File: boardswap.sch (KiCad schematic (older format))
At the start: 154 parts, among them J1 USB_C_Receptacle_USB2.0, SW1 SW_Push, U1 ATmega32U4-AU, Y1 16MHz

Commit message: did most placement
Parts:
- C7: footprint Diode_SMD:D_SOD-123 -> Capacitor_SMD:C_0805_2012Metric
- J1: footprint keyswitches:Kailh_socket_MX -> Connector_USB:USB_C_Receptacle_HRO_TYPE-C-31-M-12
- U1: footprint Package_QFP:TQFP-44_10x10mm_P0.8mm -> Package_DFN_QFN:QFN-44-1EP_7x7mm_P0.5mm_EP5.2x5.2mm
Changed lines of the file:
@@
 F 0 "J1" H 1307 7367 50  0000 C CNN
 F 1 "USB_C_Receptacle_USB2.0" H 1307 7276 50  0000 C CNN
-F 2 "keyswitches:Kailh_socket_MX" H 1350 6500 50  0001 C CNN
+F 2 "Connector_USB:USB_C_Receptacle_HRO_TYPE-C-31-M-12" H 1350 6500 50  0001 C CNN
 F 3 "https://www.usb.org/sites/default/files/documents/usb_type-c.zip" H 1350 6500 50  0001 C CNN
 	1    1200 6500
@@
 F 0 "C7" H 2042 3746 50  0000 L CNN
 F 1 "10uF" H 2042 3655 50  0000 L CNN
-F 2 "Diode_SMD:D_SOD-123" H 1950 3700 50  0001 C CNN
+F 2 "Capacitor_SMD:C_0805_2012Metric" H 1950 3700 50  0001 C CNN
 F 3 "~" H 1950 3700 50  0001 C CNN
 	1    1950 3700
@@
 F 0 "U1" H 3400 1111 50  0000 C CNN
 F 1 "ATmega32U4-AU" H 3400 1020 50  0000 C CNN
-F 2 "Package_QFP:TQFP-44_10x10mm_P0.8mm" H 3400 3000 50  0001 C CIN
+F 2 "Package_DFN_QFN:QFN-44-1EP_7x7mm_P0.5mm_EP5.2x5.2mm" H 3400 3000 50  0001 C CIN
 F 3 "http://ww1.microchip.com/downloads/en/DeviceDoc/Atmel-7766-8-bit-AVR-ATmega16U4-32U4_Datasheet.pdf" H 3400 3000 50  0001 C CNN
 	1    3400 3000

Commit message: hewwo backups owo
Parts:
- U1: footprint Package_DFN_QFN:QFN-44-1EP_7x7mm_P0.5mm_EP5.2x5.2mm -> Package_QFP:TQFP-44_10x10mm_P0.8mm
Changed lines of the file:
@@
 F 0 "U1" H 3400 1111 50  0000 C CNN
 F 1 "ATmega32U4-AU" H 3400 1020 50  0000 C CNN
-F 2 "Package_DFN_QFN:QFN-44-1EP_7x7mm_P0.5mm_EP5.2x5.2mm" H 3400 3000 50  0001 C CIN
+F 2 "Package_QFP:TQFP-44_10x10mm_P0.8mm" H 3400 3000 50  0001 C CIN
 F 3 "http://ww1.microchip.com/downloads/en/DeviceDoc/Atmel-7766-8-bit-AVR-ATmega16U4-32U4_Datasheet.pdf" H 3400 3000 50  0001 C CNN
 	1    3400 3000

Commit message: placed components
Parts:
- C4, C5, C6, C7: footprint Capacitor_SMD:C_0805_2012Metric -> Capacitor_SMD:C_0603_1608Metric
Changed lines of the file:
@@
 	1    0    0    -1
 $EndComp
-Connection ~ 2800 1500
 Wire Wire Line
 	2300 1500 2300 1200
@@
 	1    0    0    -1
 $EndComp
-Wire Wire Line
-	2800 1500 2800 1250
 $Comp
 L Device:R_Small R1
@@
 F 0 "C7" H 2042 3746 50  0000 L CNN
 F 1 "10uF" H 2042 3655 50  0000 L CNN
-F 2 "Capacitor_SMD:C_0805_2012Metric" H 1950 3700 50  0001 C CNN
+F 2 "Capacitor_SMD:C_0603_1608Metric" H 1950 3700 50  0001 C CNN
 F 3 "~" H 1950 3700 50  0001 C CNN
 	1    1950 3700
@@
 F 0 "C6" H 1642 3746 50  0000 L CNN
 F 1 "0.1uF" H 1642 3655 50  0000 L CNN
-F 2 "Capacitor_SMD:C_0805_2012Metric" H 1550 3700 50  0001 C CNN
+F 2 "Capacitor_SMD:C_0603_1608Metric" H 1550 3700 50  0001 C CNN
 F 3 "~" H 1550 3700 50  0001 C CNN
 	1    1550 3700
@@
 F 0 "C5" H 1242 3746 50  0000 L CNN
 F 1 "0.1uF" H 1242 3655 50  0000 L CNN
-F 2 "Capacitor_SMD:C_0805_2012Metric" H 1150 3700 50  0001 C CNN
+F 2 "Capacitor_SMD:C_0603_1608Metric" H 1150 3700 50  0001 C CNN
 F 3 "~" H 1150 3700 50  0001 C CNN
 	1    1150 3700
@@
 F 0 "C4" H 842 3746 50  0000 L CNN
 F 1 "0.1uF" H 842 3655 50  0000 L CNN
-F 2 "Capacitor_SMD:C_0805_2012Metric" H 750 3700 50  0001 C CNN
+F 2 "Capacitor_SMD:C_0603_1608Metric" H 750 3700 50  0001 C CNN
 F 3 "~" H 750 3700 50  0001 C CNN
 	1    750  3700
@@
 $EndComp
 Wire Wire Line
-	3300 4800 2950 4800
-Connection ~ 3300 4800
-Wire Wire Line
-	2950 4800 2950 4900
-Wire Wire Line
-	3400 4800 3300 4800
-$Comp
-L power:GND #PWR0109
-U 1 1 5F31D09C
-P 2950 4900
-F 0 "#PWR0109" H 2950 4650 50  0001 C CNN
-F 1 "GND" H 2955 4727 50  0000 C CNN
-F 2 "" H 2950 4900 50  0001 C CNN
-F 3 "" H 2950 4900 50  0001 C CNN
-	1    2950 4900
-	1    0    0    -1
-$EndComp
-Wire Wire Line
-	3400 1200 3400 1050
-Wire Wire Line
 	3400 1200 3500 1200
 Connection ~ 3400 1200
@@
 F 3 "" H 3400 1050 50  0001 C CNN
 	1    3400 1050
-	1    0    0    -1
-$EndComp
-$Comp
-L MCU_Microchip_ATmega:ATmega32U4-AU U1
-U 1 1 5F319131
-P 3400 3000
-F 0 "U1" H 3400 1111 50  0000 C CNN
-F 1 "ATmega32U4-AU" H 3400 1020 50  0000 C CNN
-F 2 "Package_QFP:TQFP-44_10x10mm_P0.8mm" H 3400 3000 50  0001 C CIN
-F 3 "http://ww1.microchip.com/downloads/en/DeviceDoc/Atmel-7766-8-bit-AVR-ATmega16U4-32U4_Datasheet.pdf" H 3400 3000 50  0001 C CNN
-	1    3400 3000
 	1    0    0    -1
 $EndComp
@@
 Text GLabel 10500 1200 1    50   Input ~ 0
 COL13
+Wire Wire Line
+	3400 1200 3400 1050
+Wire Wire Line
+	2800 1500 2800 1250
+$Comp
+L power:GND #PWR0109
+U 1 1 5F31D09C
+P 2950 4900
+F 0 "#PWR0109" H 2950 4650 50  0001 C CNN
+F 1 "GND" H 2955 4727 50  0000 C CNN
+F 2 "" H 2950 4900 50  0001 C CNN
+F 3 "" H 2950 4900 50  0001 C CNN
+	1    2950 4900
+	1    0    0    -1
+$EndComp
+Connection ~ 2800 1500
+Wire Wire Line
+	2950 4800 2950 4900
+$Comp
+L MCU_Microchip_ATmega:ATmega32U4-AU U1
+U 1 1 5F319131
+P 3400 3000
+F 0 "U1" H 3400 1111 50  0000 C CNN
+F 1 "ATmega32U4-AU" H 3400 1020 50  0000 C CNN
+F 2 "Package_QFP:TQFP-44_10x10mm_P0.8mm" H 3400 3000 50  0001 C CIN
+F 3 "http://ww1.microchip.com/downloads/en/DeviceDoc/Atmel-7766-8-bit-AVR-ATmega16U4-32U4_Datasheet.pdf" H 3400 3000 50  0001 C CNN
+	1    3400 3000
+	1    0    0    -1
+$EndComp
+Wire Wire Line
+	3400 4800 3300 4800
+Connection ~ 3300 4800
+Wire Wire Line
+	2950 4800 3300 4800
 $EndSCHEMATC

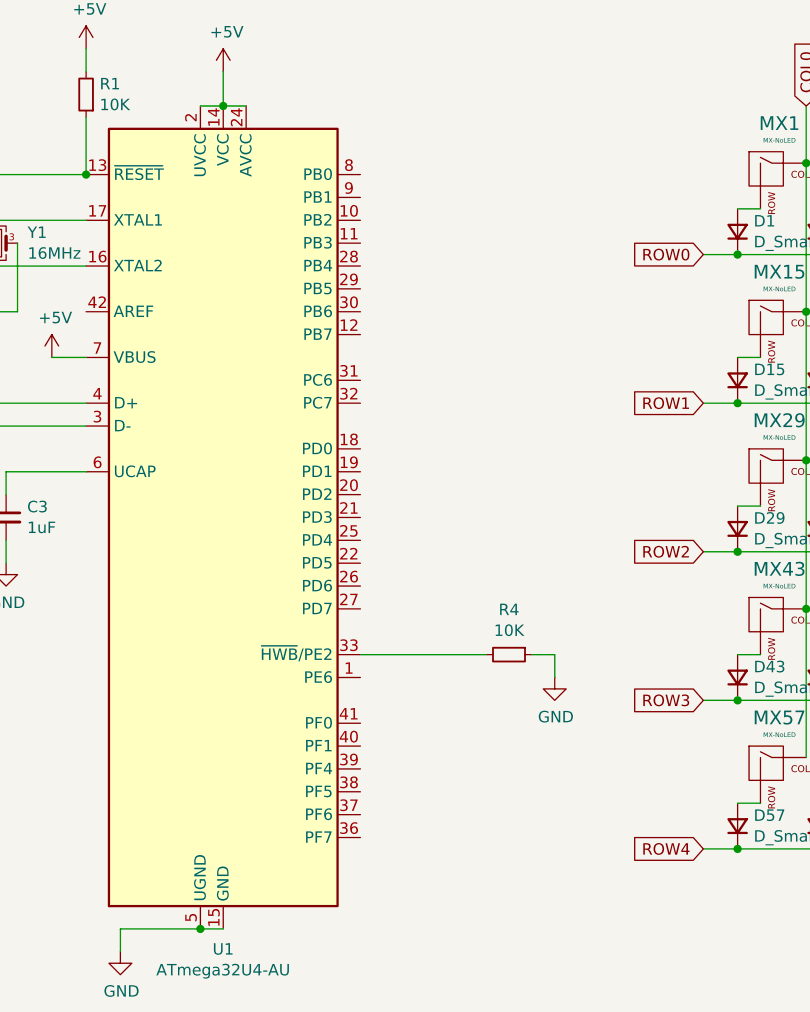
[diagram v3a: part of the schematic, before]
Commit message: done routing probably
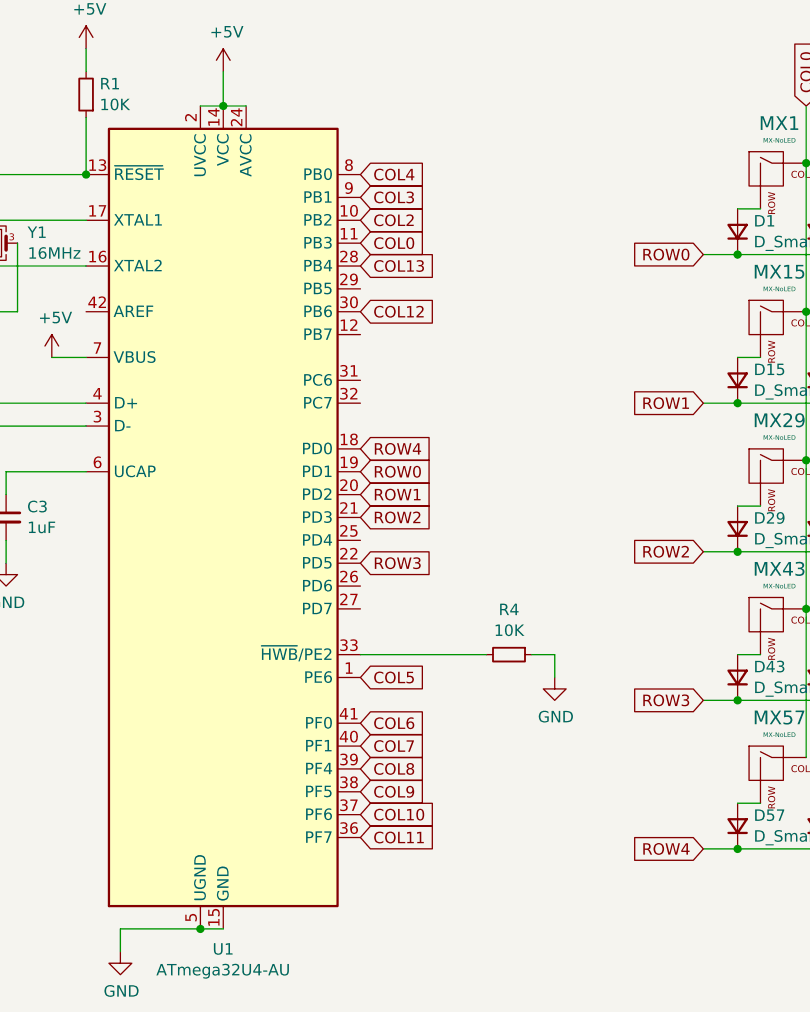
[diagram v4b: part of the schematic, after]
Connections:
- net COL0: now also U1.11 (PB3)
- net COL10: now also U1.37 (PF6)
- net COL11: now also U1.36 (PF7)
- net COL12: now also U1.30 (PB6)
- net COL13: now also U1.28 (PB4)
- net COL2: now also U1.10 (PB2)
- net COL3: now also U1.9 (PB1)
- net COL4: now also U1.8 (PB0)
- net COL5: now also U1.1 (PE6)
- net COL6: now also U1.41 (PF0)
- net COL7: now also U1.40 (PF1)
- net COL8: now also U1.39 (PF4)
- net COL9: now also U1.38 (PF5)
- net ROW0: now also U1.19 (PD1)
- net ROW1: now also U1.20 (PD2)
- net ROW2: now also U1.21 (PD3)
- net ROW3: now also U1.22 (PD5)
- net ROW4: now also U1.18 (PD0)
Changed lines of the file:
@@
 Wire Wire Line
 	2950 4800 3300 4800
+Text GLabel 4000 3200 2    50   Input ~ 0
+ROW3
+Text GLabel 4000 3000 2    50   Input ~ 0
+ROW2
+Text GLabel 4000 2900 2    50   Input ~ 0
+ROW1
+Text GLabel 4000 2800 2    50   Input ~ 0
+ROW0
+Text GLabel 4000 2700 2    50   Input ~ 0
+ROW4
+Text GLabel 4000 1800 2    50   Input ~ 0
+COL0
+Text GLabel 4000 1700 2    50   Input ~ 0
+COL2
+Text GLabel 4000 1600 2    50   Input ~ 0
+COL3
+Text GLabel 4000 1500 2    50   Input ~ 0
+COL4
+Text GLabel 4000 3700 2    50   Input ~ 0
+COL5
+Text GLabel 4000 3900 2    50   Input ~ 0
+COL6
+Text GLabel 4000 4000 2    50   Input ~ 0
+COL7
+Text GLabel 4000 4100 2    50   Input ~ 0
+COL8
+Text GLabel 4000 4200 2    50   Input ~ 0
+COL9
+Text GLabel 4000 4300 2    50   Input ~ 0
+COL10
+Text GLabel 4000 4400 2    50   Input ~ 0
+COL11
+Text GLabel 4000 2100 2    50   Input ~ 0
+COL12
+Text GLabel 4000 1900 2    50   Input ~ 0
+COL13
 $EndSCHEMATC

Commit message: rotated mcu, begrudgingly
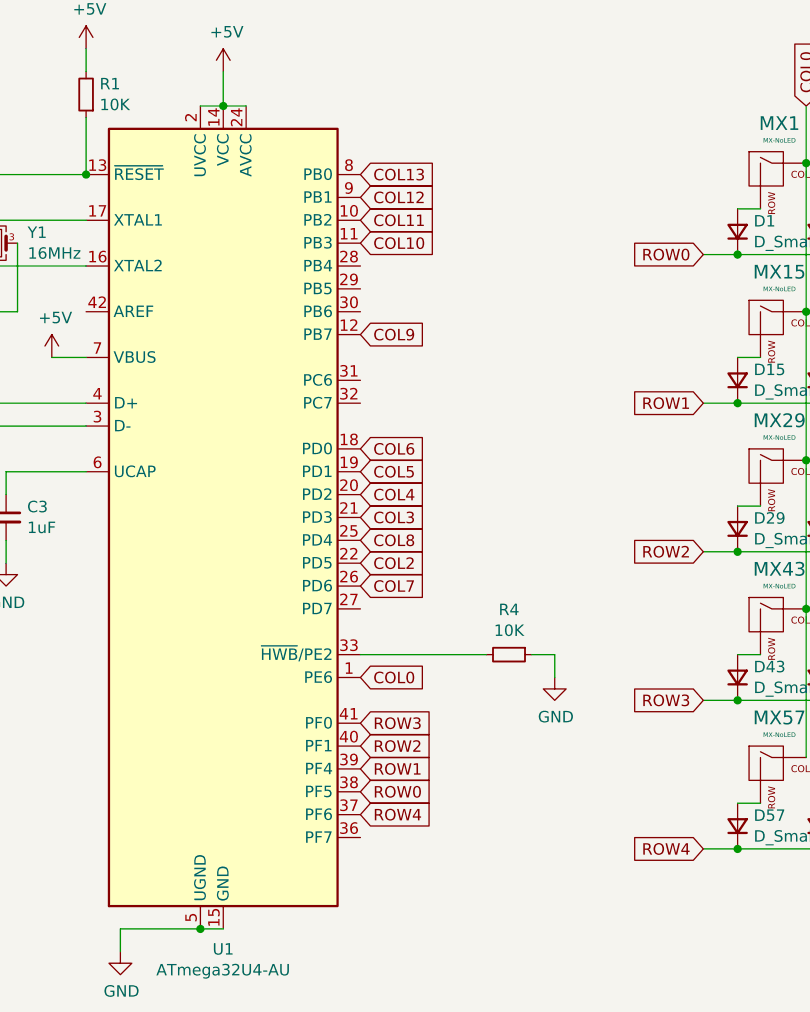
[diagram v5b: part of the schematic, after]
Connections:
- net COL0: now also U1.1 (PE6); no longer U1.11 (PB3)
- net COL10: now also U1.11 (PB3); no longer U1.37 (PF6)
- net COL11: now also U1.10 (PB2); no longer U1.36 (PF7)
- net COL12: now also U1.9 (PB1); no longer U1.30 (PB6)
- net COL13: now also U1.8 (PB0); no longer U1.28 (PB4)
- net COL2: now also U1.22 (PD5); no longer U1.10 (PB2)
- net COL3: now also U1.21 (PD3); no longer U1.9 (PB1)
- net COL4: now also U1.20 (PD2); no longer U1.8 (PB0)
- net COL5: now also U1.19 (PD1); no longer U1.1 (PE6)
- net COL6: now also U1.18 (PD0); no longer U1.41 (PF0)
- net COL7: now also U1.26 (PD6); no longer U1.40 (PF1)
- net COL8: now also U1.25 (PD4); no longer U1.39 (PF4)
- net COL9: now also U1.12 (PB7); no longer U1.38 (PF5)
- net ROW0: now also U1.38 (PF5); no longer U1.19 (PD1)
- net ROW1: now also U1.39 (PF4); no longer U1.20 (PD2)
- net ROW2: now also U1.40 (PF1); no longer U1.21 (PD3)
- net ROW3: now also U1.41 (PF0); no longer U1.22 (PD5)
- net ROW4: now also U1.37 (PF6); no longer U1.18 (PD0)
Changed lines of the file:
@@
 Wire Wire Line
 	2800 2800 2450 2800
-$Comp
-L Device:C_Small C3
-U 1 1 5F32256C
-P 2450 3000
-F 0 "C3" H 2542 3046 50  0000 L CNN
-F 1 "1uF" H 2542 2955 50  0000 L CNN
-F 2 "Capacitor_SMD:C_0805_2012Metric" H 2450 3000 50  0001 C CNN
-F 3 "~" H 2450 3000 50  0001 C CNN
-	1    2450 3000
-	1    0    0    -1
-$EndComp
 Wire Wire Line
 	1550 2600 1400 2600
@@
 Wire Wire Line
 	2950 4800 3300 4800
+Text GLabel 4000 3900 2    50   Input ~ 0
+ROW3
+Text GLabel 4000 4000 2    50   Input ~ 0
+ROW2
+Text GLabel 4000 4100 2    50   Input ~ 0
+ROW1
+Text GLabel 4000 4200 2    50   Input ~ 0
+ROW0
+Text GLabel 4000 4300 2    50   Input ~ 0
+ROW4
+Text GLabel 4000 3700 2    50   Input ~ 0
+COL0
+Text GLabel 4000 3000 2    50   Input ~ 0
+COL3
+Text GLabel 4000 2900 2    50   Input ~ 0
+COL4
+Text GLabel 4000 2800 2    50   Input ~ 0
+COL5
+Text GLabel 4000 2700 2    50   Input ~ 0
+COL6
+Text GLabel 4000 3300 2    50   Input ~ 0
+COL7
+Text GLabel 4000 3100 2    50   Input ~ 0
+COL8
+Text GLabel 4000 2200 2    50   Input ~ 0
+COL9
+Text GLabel 4000 1800 2    50   Input ~ 0
+COL10
+Text GLabel 4000 1700 2    50   Input ~ 0
+COL11
+Text GLabel 4000 1600 2    50   Input ~ 0
+COL12
+Text GLabel 4000 1500 2    50   Input ~ 0
+COL13
+$Comp
+L Device:C_Small C3
+U 1 1 5F32256C
+P 2450 3000
+F 0 "C3" H 2542 3046 50  0000 L CNN
+F 1 "1uF" H 2542 2955 50  0000 L CNN
+F 2 "Capacitor_SMD:C_0805_2012Metric" H 2450 3000 50  0001 C CNN
+F 3 "~" H 2450 3000 50  0001 C CNN
+	1    2450 3000
+	1    0    0    -1
+$EndComp
 Text GLabel 4000 3200 2    50   Input ~ 0
-ROW3
-Text GLabel 4000 3000 2    50   Input ~ 0
-ROW2
-Text GLabel 4000 2900 2    50   Input ~ 0
-ROW1
-Text GLabel 4000 2800 2    50   Input ~ 0
-ROW0
-Text GLabel 4000 2700 2    50   Input ~ 0
-ROW4
-Text GLabel 4000 1800 2    50   Input ~ 0
-COL0
-Text GLabel 4000 1700 2    50   Input ~ 0
 COL2
-Text GLabel 4000 1600 2    50   Input ~ 0
-COL3
-Text GLabel 4000 1500 2    50   Input ~ 0
-COL4
-Text GLabel 4000 3700 2    50   Input ~ 0
-COL5
-Text GLabel 4000 3900 2    50   Input ~ 0
-COL6
-Text GLabel 4000 4000 2    50   Input ~ 0
-COL7
-Text GLabel 4000 4100 2    50   Input ~ 0
-COL8
-Text GLabel 4000 4200 2    50   Input ~ 0
-COL9
-Text GLabel 4000 4300 2    50   Input ~ 0
-COL10
-Text GLabel 4000 4400 2    50   Input ~ 0
-COL11
-Text GLabel 4000 2100 2    50   Input ~ 0
-COL12
-Text GLabel 4000 1900 2    50   Input ~ 0
-COL13
 $EndSCHEMATC
